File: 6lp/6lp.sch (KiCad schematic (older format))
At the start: 34 parts, among them J1 MODULE_HEADER, T1 2450BM15A0015, U1 AT86RF233, X1 16.0000MF09Z-AC3

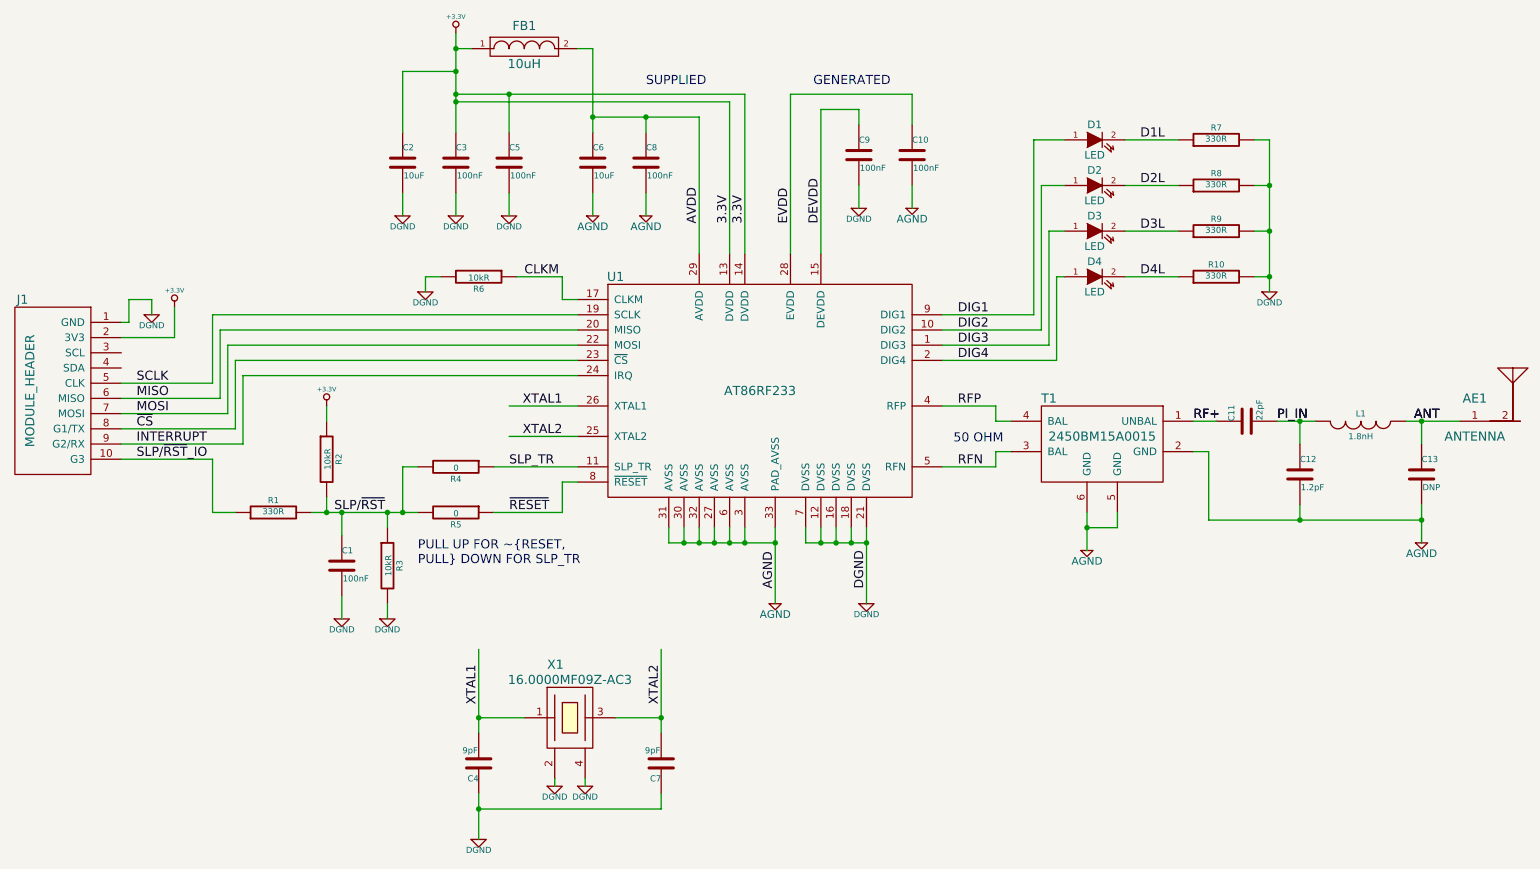
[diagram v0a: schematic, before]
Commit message: closed project for review
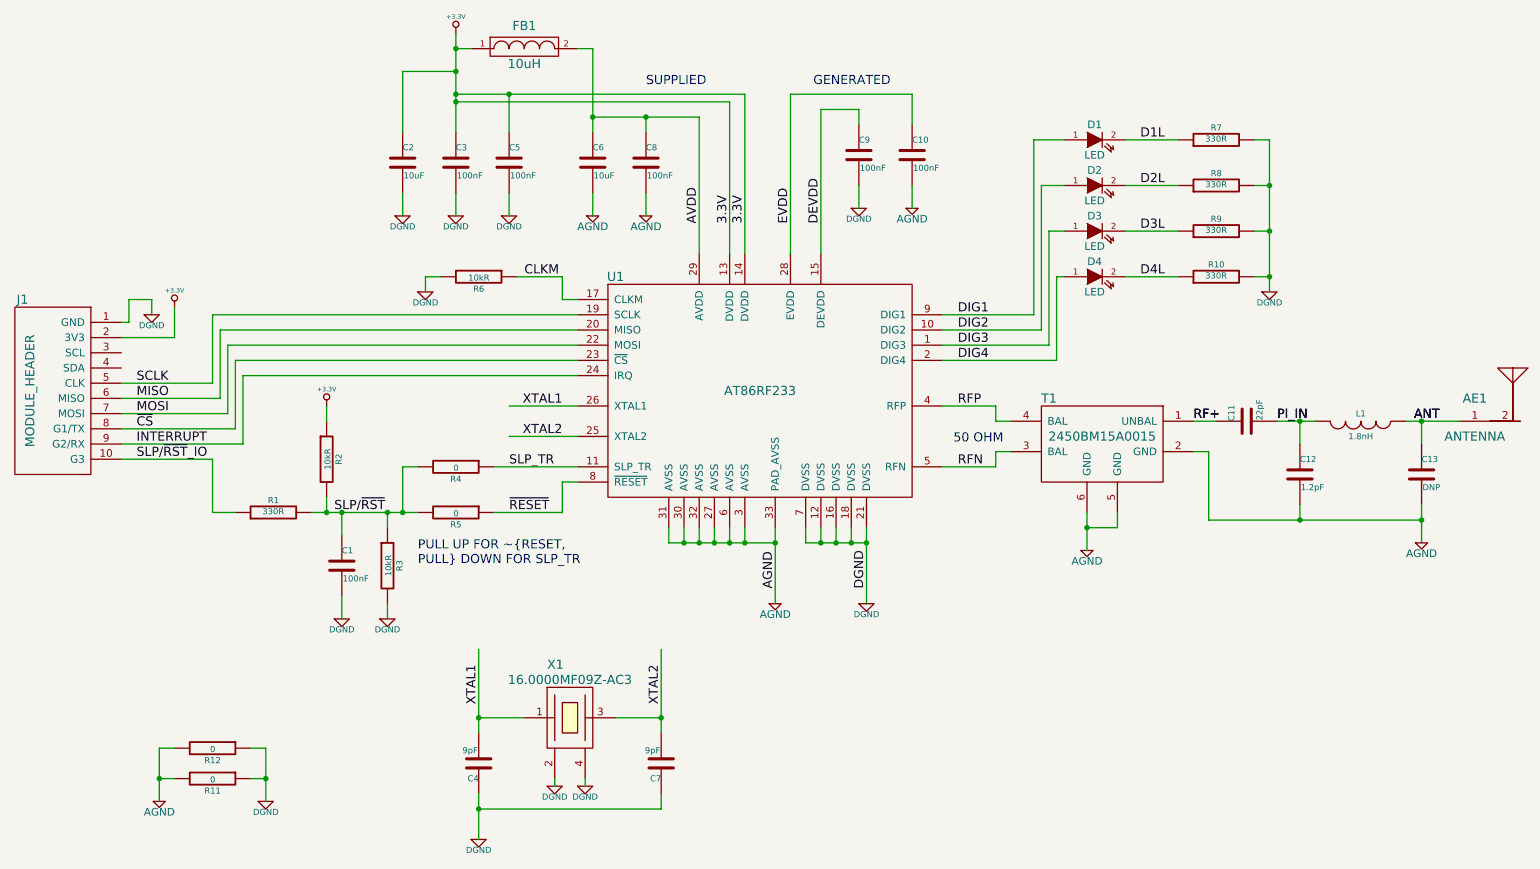
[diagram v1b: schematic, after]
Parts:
- added R11, R12: 0, Resistors_SMD:R_0402, symbol R
- T1: footprint (none) -> parts:EIA-0805
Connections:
- net AGND: now also R11.2, R12.2
- net DGND: now also R11.1, R12.1
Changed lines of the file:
@@
 SLP_TR
 Wire Wire Line
-	6000 4550 6000 4650
-Wire Wire Line
-	6000 4650 6000 5050
-Wire Wire Line
-	5300 4650 5400 4650
-Wire Wire Line
-	5400 4650 5500 4650
-Wire Wire Line
-	5500 4650 5600 4650
-Wire Wire Line
-	5600 4650 5700 4650
-Wire Wire Line
-	5700 4650 5800 4650
-Wire Wire Line
-	5800 4650 6000 4650
+	6000 4550 6000 5050
+Wire Wire Line
+	5300 4650 6000 4650
 Wire Wire Line
 	5700 4650 5700 4550
@@
 	6500 4650 6500 4550
 Wire Wire Line
-	6200 4650 6300 4650
-Wire Wire Line
-	6300 4650 6400 4650
-Wire Wire Line
-	6400 4650 6500 4650
-Wire Wire Line
-	6500 4650 6600 4650
-Wire Wire Line
-	6600 4550 6600 4650
-Wire Wire Line
-	6600 4650 6600 5050
+	6200 4650 6600 4650
+Wire Wire Line
+	6600 4550 6600 5050
 Connection ~ 6600 4650
 Wire Wire Line
@@
 	6100 1700 6100 2750
 Wire Wire Line
-	3900 1300 3900 1400
-Wire Wire Line
-	3900 1400 3900 1550
-Wire Wire Line
-	3900 1550 3900 1700
-Wire Wire Line
-	3900 1700 3900 1750
-Wire Wire Line
-	3900 1750 3900 1950
-Wire Wire Line
-	4800 1850 5150 1850
-Wire Wire Line
-	5150 1850 5500 1850
+	3900 1300 3900 1950
+Wire Wire Line
+	4800 1850 5500 1850
 Wire Wire Line
 	5700 1750 5700 2750
@@
 	4800 2350 4800 2500
 Wire Wire Line
-	4800 1400 4800 1850
-Wire Wire Line
-	4800 1850 4800 1950
+	4800 1400 4800 1950
 Connection ~ 4800 1850
 Wire Wire Line
@@
 Connection ~ 3900 1750
 Wire Wire Line
-	3900 1700 4250 1700
-Wire Wire Line
-	4250 1700 5800 1700
+	3900 1700 5800 1700
 Wire Wire Line
 	3550 2500 3550 2350
@@
 	3050 3750 3050 3850
 Wire Wire Line
-	4050 6300 4050 6400
-Wire Wire Line
-	4050 6400 4050 6600
+	4050 6300 4050 6600
 Wire Wire Line
 	4050 6400 5250 6400
@@
 	4600 4250 4700 4250
 Wire Wire Line
-	5250 5350 5250 5800
-Wire Wire Line
-	5250 5800 5250 5900
+	5250 5350 5250 5900
 Wire Wire Line
 	4050 5800 4350 5800
@@
 Connection ~ 4250 1700
 Wire Wire Line
-	10150 3850 10250 3850
-Wire Wire Line
-	10250 3850 10500 3850
+	10150 3850 10500 3850
 Wire Wire Line
 	10250 4000 10250 3850
 Connection ~ 10250 3850
 Wire Wire Line
-	9300 3850 9450 3850
-Wire Wire Line
-	9450 3850 9550 3850
+	9300 3850 9550 3850
 Wire Wire Line
 	9450 4000 9450 3850
@@
 	8850 4050 8850 4500
 Wire Wire Line
-	8850 4500 9450 4500
-Wire Wire Line
-	9450 4500 10250 4500
-Wire Wire Line
-	10250 4400 10250 4500
-Wire Wire Line
-	10250 4500 10250 4650
+	8850 4500 10250 4500
+Wire Wire Line
+	10250 4400 10250 4650
 Wire Wire Line
 	9450 4400 9450 4500
@@
 	8750 4050 8850 4050
 Wire Wire Line
-	8050 4450 8050 4550
-Wire Wire Line
-	8050 4550 8050 4700
+	8050 4450 8050 4700
 Wire Wire Line
 	8050 4550 8250 4550
@@
 Connection ~ 5600 4650
 Wire Wire Line
-	4050 5350 4050 5800
-Wire Wire Line
-	4050 5800 4050 5900
+	4050 5350 4050 5900
 Wire Wire Line
 	2500 4000 2500 3550
@@
 	8300 2900 8650 2900
 Wire Wire Line
-	9250 2000 9250 2300
-Wire Wire Line
-	9250 2300 9250 2600
-Wire Wire Line
-	9250 2600 9250 2900
-Wire Wire Line
-	9250 2900 9250 3000
+	9250 2000 9250 3000
 Wire Wire Line
 	9250 2900 9150 2900
@@
 	4150 4150 4700 4150
 Wire Wire Line
-	2950 4450 3050 4450
-Wire Wire Line
-	3050 4450 3150 4450
-Wire Wire Line
-	3150 4450 3450 4450
-Wire Wire Line
-	3450 4450 3550 4450
-Wire Wire Line
-	3550 4450 3650 4450
+	2950 4450 3650 4450
 Wire Wire Line
 	4150 4450 4600 4450
@@
 F 0 "T1" H 8500 4200 60  0000 C CNN
 F 1 "2450BM15A0015" H 8150 3950 60  0000 C CNN
-F 2 "" H 8150 3950 60  0000 C CNN
+F 2 "parts:EIA-0805" H 8150 3950 60  0001 C CNN
 F 3 "" H 8150 3950 60  0000 C CNN
 	1    8150 3950
 	-1   0    0    -1
 $EndComp
+$Comp
+L AGND #PWR023
+U 1 1 543E1BA0
+P 1950 6350
+F 0 "#PWR023" H 1950 6350 40  0001 C CNN
+F 1 "AGND" H 1950 6280 50  0000 C CNN
+F 2 "" H 1950 6350 60  0000 C CNN
+F 3 "" H 1950 6350 60  0000 C CNN
+	1    1950 6350
+	1    0    0    -1
+$EndComp
+$Comp
+L DGND #PWR024
+U 1 1 543E1BA6
+P 2650 6350
+F 0 "#PWR024" H 2650 6350 40  0001 C CNN
+F 1 "DGND" H 2650 6280 40  0000 C CNN
+F 2 "" H 2650 6350 60  0000 C CNN
+F 3 "" H 2650 6350 60  0000 C CNN
+	1    2650 6350
+	1    0    0    -1
+$EndComp
+$Comp
+L R R11
+U 1 1 543E20DC
+P 2300 6200
+F 0 "R11" V 2380 6200 40  0000 C CNN
+F 1 "0" V 2307 6201 40  0000 C CNN
+F 2 "Resistors_SMD:R_0402" V 2230 6200 30  0001 C CNN
+F 3 "" H 2300 6200 30  0000 C CNN
+	1    2300 6200
+	0    1    1    0
+$EndComp
+Wire Wire Line
+	2550 6200 2650 6200
+Wire Wire Line
+	2650 6000 2650 6350
+Wire Wire Line
+	2050 6200 1950 6200
+Wire Wire Line
+	1950 6000 1950 6350
+$Comp
+L R R12
+U 1 1 543E311A
+P 2300 6000
+F 0 "R12" V 2380 6000 40  0000 C CNN
+F 1 "0" V 2307 6001 40  0000 C CNN
+F 2 "Resistors_SMD:R_0402" V 2230 6000 30  0001 C CNN
+F 3 "" H 2300 6000 30  0000 C CNN
+	1    2300 6000
+	0    1    1    0
+$EndComp
+Wire Wire Line
+	2550 6000 2650 6000
+Wire Wire Line
+	2050 6000 1950 6000
+Connection ~ 2650 6200
+Connection ~ 1950 6200
 $EndSCHEMATC
